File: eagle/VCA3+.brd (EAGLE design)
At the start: 100 x 80 mm, 51 parts, among them IC1 TL072P, IC2 TL072P, Q1 2N3906, T2 2N3904, T3 2N3904, T4 2N3904, T5 2N3904, T6 2N3904

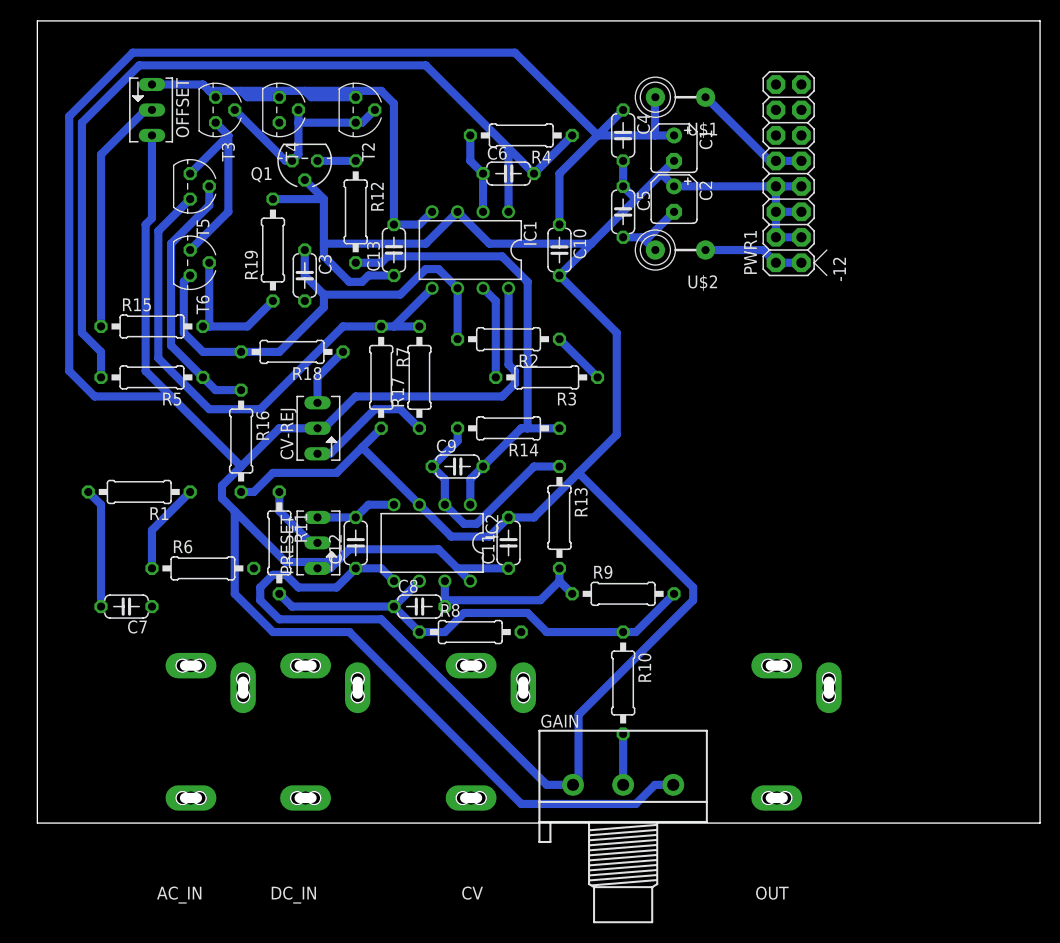
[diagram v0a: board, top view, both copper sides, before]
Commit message: routed
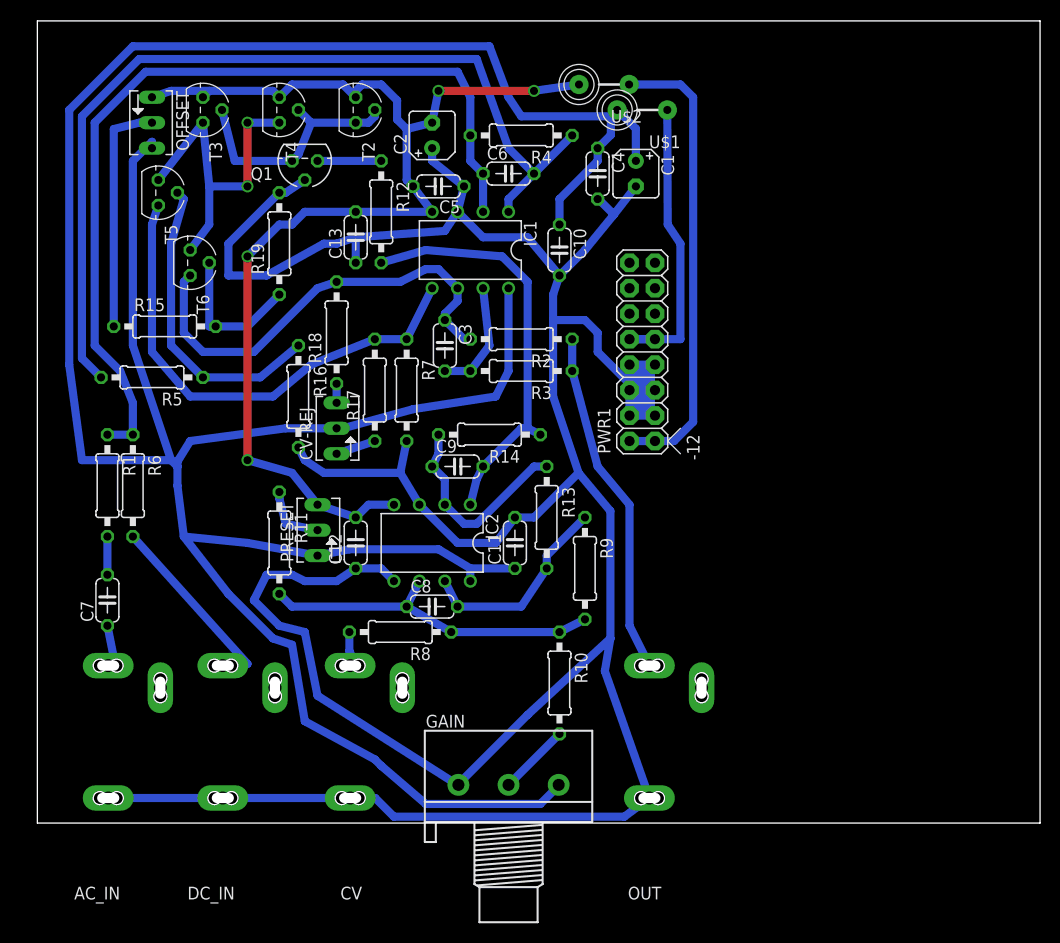
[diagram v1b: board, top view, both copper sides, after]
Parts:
- moved C2 25.0 mm to (39.4, 68.6), turned to 90 degrees
- moved PWR1 23.0 mm to (60.3, 44.5)
- moved C5 18.6 mm to (40.0, 63.5), turned to 180 degrees
- moved U$2 18.2 mm to (56.5, 73.7)
- moved C3 15.6 mm to (40.6, 47.6)
- moved OUT 12.7 mm to (66.0, 0.00)
- moved CV 12.1 mm to (36.2, 0.00)
- moved GAIN 11.4 mm to (47.0, 3.81)
- moved R6 10.8 mm to (9.53, 33.7), turned to 270 degrees
- moved AC_IN 8.26 mm to (12.1, 0.00)
- moved DC_IN 8.25 mm to (23.5, 0.00)
- moved R16 7.24 mm to (26.0, 42.5)
- moved R8 6.98 mm to (36.2, 19.1), turned to 180 degrees
- moved R10 6.35 mm to (52.1, 14.0)
- moved R18 4.84 mm to (29.8, 48.9), turned to 90 degrees
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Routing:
- net N$7: track 17.3 -> 88.0 mm
- net GND: track 261.3 -> 319.0 mm
- net -12V: track 67.7 -> 118.3 mm, vias 0 -> 4
- net N$2: track 10.1 -> 46.4 mm
- net N$6: track 5.39 -> 34.3 mm
- net N$14: track 0.00 -> 19.6 mm
- net N$1: track 12.2 -> 30.9 mm
- net N$20: track 20.2 -> 33.9 mm, vias 0 -> 2
- net N$11: track 47.7 -> 34.8 mm
- net N$26: track 12.8 -> 4.02 mm
- net N$4: track 12.0 -> 3.81 mm
- net N$3: track 0.00 -> 6.62 mm
- net N$9: track 54.1 -> 49.5 mm
- net N$18: track 46.6 -> 41.9 mm
- net N$22: track 26.3 -> 30.8 mm
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
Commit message: cutout
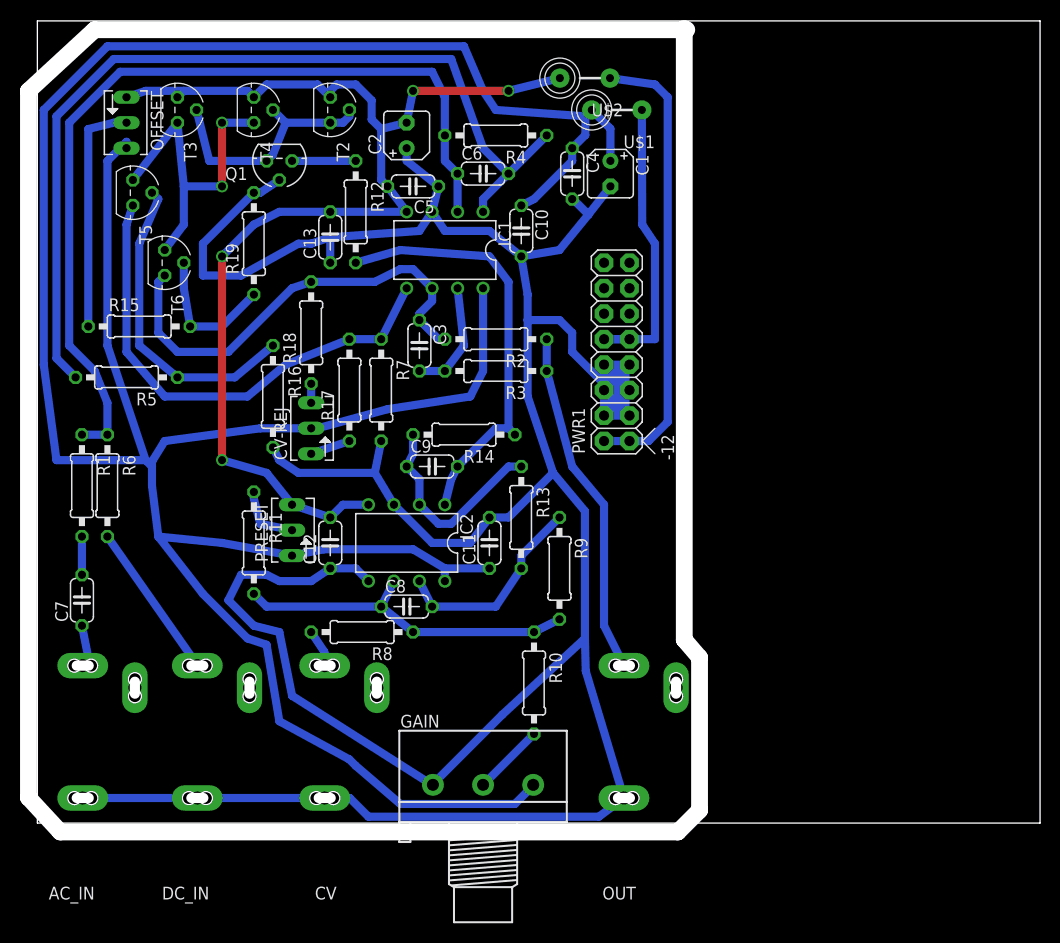
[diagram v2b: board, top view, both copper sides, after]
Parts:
- moved C10 4.26 mm to (48.3, 59.1)
- moved R8 3.81 mm to (32.4, 19.1)
- moved OUT 2.54 mm to (63.5, 0.00)
- moved PWR1 2.54 mm to (57.8, 44.5)
- moved U$1 2.54 mm to (57.8, 71.1)
- moved DC_IN 2.54 mm to (21.0, 0.00)
- moved PRESET 2.54 mm to (25.4, 29.2)
- moved Q1 2.54 mm to (24.1, 66.0)
- moved R17 2.54 mm to (31.1, 43.2)
- moved T3 2.54 mm to (14.0, 71.1)
- moved T6 2.54 mm to (12.7, 55.9)
- moved C7 2.54 mm to (4.45, 22.2)
- moved R1 2.54 mm to (4.45, 33.7)
- moved R6 2.54 mm to (6.99, 33.7)
- moved AC_IN 2.54 mm to (9.53, 0.00)
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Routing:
- net +12V: track 298.6 -> 296.9 mm
- net N$18: track 41.9 -> 42.9 mm
- net N$22: track 30.8 -> 31.5 mm
- net N$2: track 46.4 -> 45.8 mm
- net N$24: track 14.7 -> 14.1 mm
- net -12V: track 118.3 -> 118.8 mm
- net N$14: track 19.6 -> 19.1 mm
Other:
- board size 100 x 80 mm -> 100.9 x 80.9 mm
